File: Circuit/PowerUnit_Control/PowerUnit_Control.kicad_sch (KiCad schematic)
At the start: 25 parts, among them J1 Conn_01x02_Pin, J10 Conn_01x02_Pin, J11 Conn_01x02_Pin, J2 Conn_01x02_Pin, J3 Conn_01x07_Socket, J4 Conn_01x02_Pin, J5 Conn_01x02_Pin, J6 Conn_01x07_Socket, J7 Conn_01x02_Pin, J8 Conn_01x02_Pin, J9 Conn_01x07_Socket, SW1 SW_Toggle_DPDT

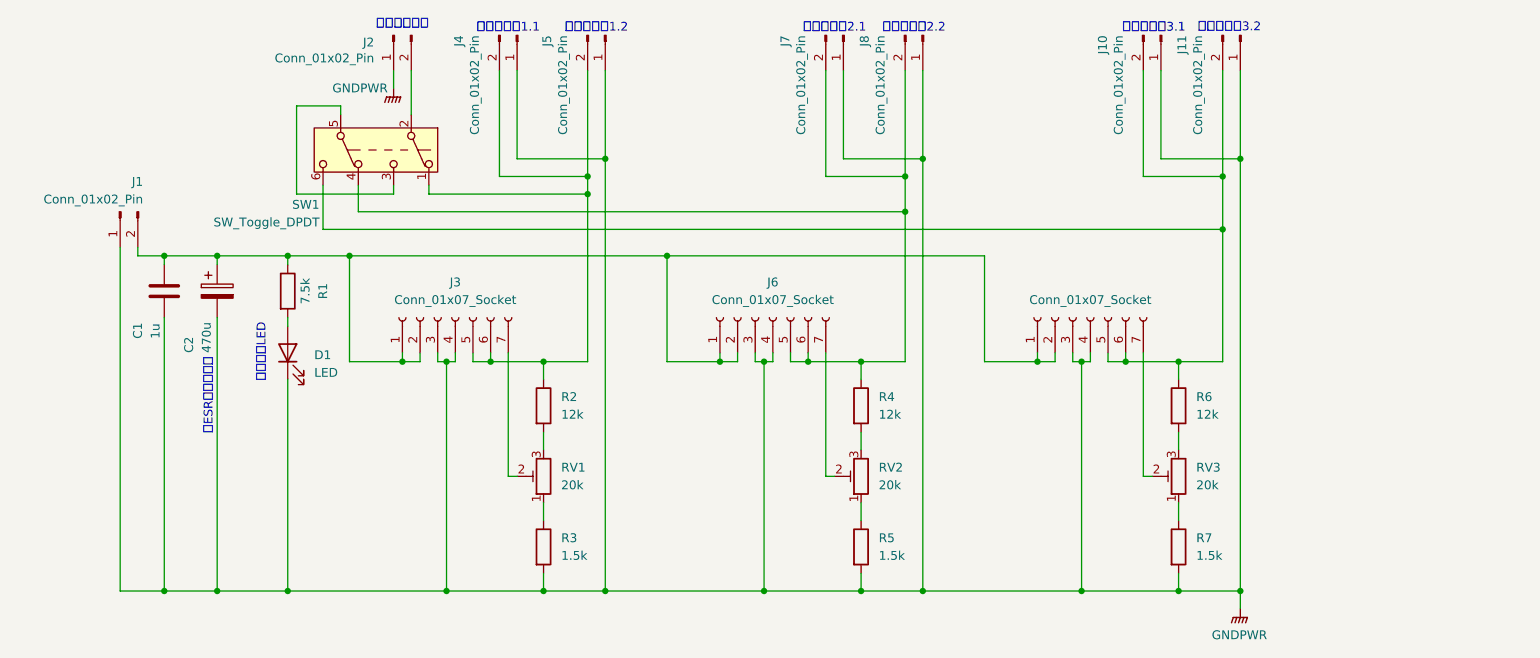
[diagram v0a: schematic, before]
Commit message: 制御電源基板が完成
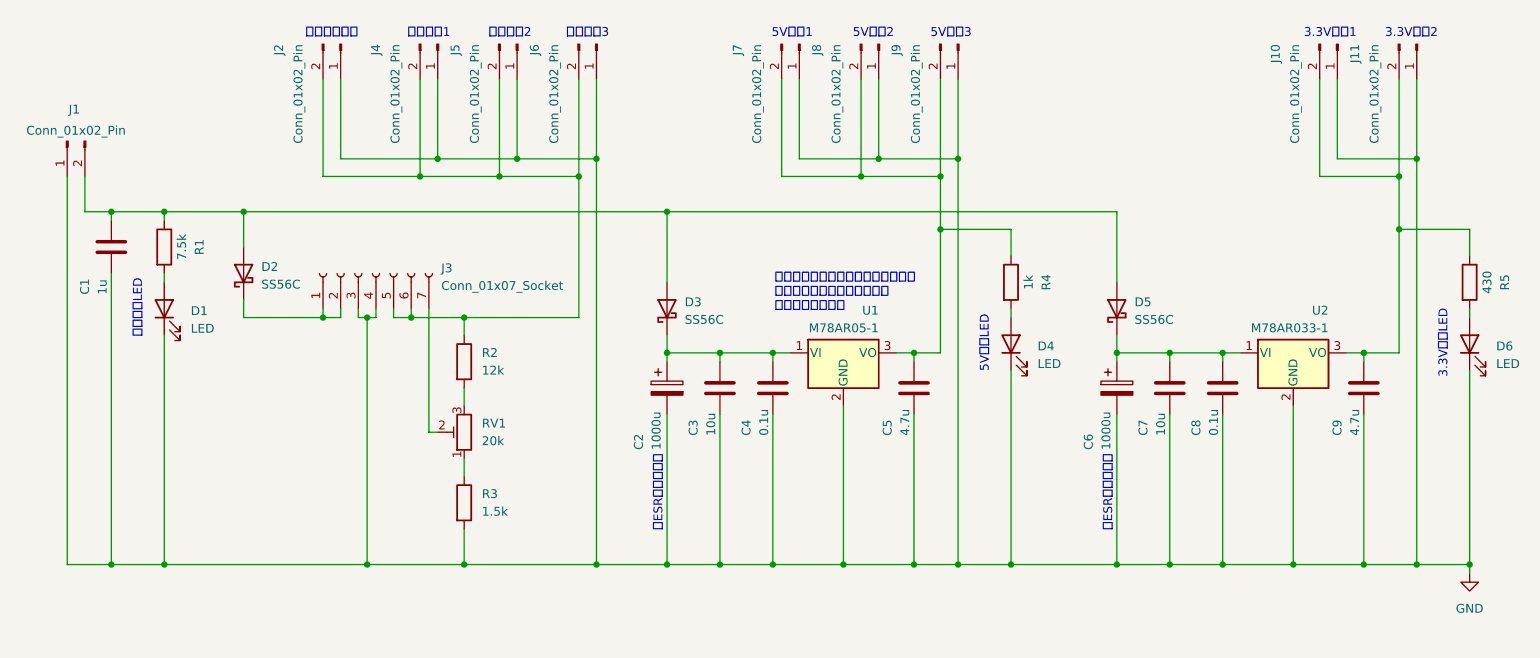
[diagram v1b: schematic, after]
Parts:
- removed J6, J9: Conn_01x07_Socket, OU_Power:YDS512F-Unit, symbol Connector:Conn_01x07_Socket
- removed R6: 12k, Resistor_THT:R_Axial_DIN0207_L6.3mm_D2.5mm_P2.54mm_Vertical, symbol Device:R
- removed R7: 1.5k, Resistor_THT:R_Axial_DIN0207_L6.3mm_D2.5mm_P2.54mm_Vertical, symbol Device:R
- removed RV2, RV3: 20k, OU_Reg:TRIM_3296W-1-250, symbol Device:R_Potentiometer_Trim
- removed SW1: SW_Toggle_DPDT, OU_Switch:1MD6-T1-B1-M1-Q-N-S, symbol Switch:SW_Push_DPDT
- added C3, C7: 10u, Capacitor_SMD:C_1206_3216Metric, symbol Device:C
- added C4, C8: 0.1u, Capacitor_SMD:C_0603_1608Metric, symbol Device:C
- added C5, C9: 4.7u, Capacitor_SMD:C_0805_2012Metric, symbol Device:C
- added C6: 1000u, Capacitor_THT:CP_Radial_D16.0mm_P7.50mm, symbol Device:C_Polarized
- added D2, D3, D5: SS56C, OU_Diode:DIODE_SS56C-HF_CIP, symbol Device:D_Schottky
- added D4, D6: LED, LED_THT:LED_D5.0mm, symbol Device:LED
- added J6: Conn_01x02_Pin, OU_Conn:AMASS_XT30U-F, symbol Connector:Conn_01x02_Pin
- added J9: Conn_01x02_Pin, OU_Conn:Hirose_DF1EC-2P-2.5DSA_1x02_P2.5mm_Vertical, symbol Connector:Conn_01x02_Pin
- added U1: M78AR05-1, OU_Power:M78AR05-1, symbol Regulator_Linear:LM7812_TO220
- added U2: M78AR033-1, OU_Power:M78AR033-1, symbol Regulator_Linear:LM7812_TO220
- C1: footprint Capacitor_THT:C_Disc_D6.0mm_W4.4mm_P5.00mm -> Capacitor_SMD:C_0603_1608Metric; MPN (none) -> C15849; MPN_URL https://akizukidenshi.com/catalog/g/g108150/ -> (none)
- C2: value 470u -> 1000u; footprint Capacitor_THT:CP_Radial_D10.0mm_P5.00mm -> Capacitor_THT:CP_Radial_D16.0mm_P7.50mm; MPN_URL https://akizukidenshi.com/catalog/g/g102719/ -> https://akizukidenshi.com/catalog/g/g108442/
- J1: footprint OU_Conn:AMASS_XT60PW-M -> OU_Conn:AMASS_XT30PW-M; MPN (none) -> XT30PW-M; MPN_URL (none) -> https://akizukidenshi.com/catalog/g/g117949/
- J10, J11, J7, J8: footprint OU_Conn:AMASS_XT30U-F -> OU_Conn:Hirose_DF1EC-2P-2.5DSA_1x02_P2.5mm_Vertical; MPN XT30PW-M -> (none); MPN_URL https://akizukidenshi.com/catalog/g/g117949/ -> (none)
- R2, R3: footprint Resistor_THT:R_Axial_DIN0207_L6.3mm_D2.5mm_P2.54mm_Vertical -> Resistor_SMD:R_0603_1608Metric
- R4: value 12k -> 1k
- R5: value 1.5k -> 430
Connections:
- net at C1.1, J1.2 (Pin_2), R1.1: now also D2.2 (A), D3.2 (A), D5.2 (A); no longer C2.1, J3.1 (Pin_1), J3.2 (Pin_2)
- net at J10.2 (Pin_2), J11.2 (Pin_2): now also R5.1, C9.1, U2.3 (VO)
- net at J7.2 (Pin_2), J8.2 (Pin_2), R4.1: now also C5.1, J9.2 (Pin_2), U1.3 (VO)
- net at J3.5 (Pin_5), J3.6 (Pin_6), J4.2 (Pin_2)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: now also J2.2 (Pin_2), J6.2 (Pin_2)
- net at R4.2: now also D4.2 (A)
- net GNDPWR renamed GND
- net GND: now also C3.2, C4.2, C5.2, C6.2, C7.2, C8.2, C9.2, D4.1 (K), D6.1 (K), J6.1 (Pin_1), J9.1 (Pin_1), U1.2 (GND), U2.2 (GND); no longer R5.2
- new net: C2.1, C3.1, C4.1, D3.1 (K), U1.1 (VI)
- new net: C6.1, C7.1, C8.1, D5.1 (K), U2.1 (VI)
- new net: D2.1 (K), J3.1 (Pin_1), J3.2 (Pin_2)
- new net: D6.2 (A), R5.2
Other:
- note added: "3.3V電源1"
- note added: "3.3V電源2"
- note added: "3.3V電源LED"
- note added: "5V電源1"
- note added: "5V電源2"
- note added: "5V電源3"
- note added: "5V電源LED"
- note added: "リニアレギュレータっぽいですが、 ピン互換があるスイッチング レギュレータです"
- note added: "制御電源LED"
- note added: "汎用電源1"
- note added: "汎用電源2"
- note added: "汎用電源3"
- note removed: "サーボ汎用1.1"
- note removed: "サーボ汎用1.2"
- note removed: "サーボ汎用2.1"
- note removed: "サーボ汎用2.2"
- note removed: "サーボ汎用3.1"
- note removed: "サーボ汎用3.2"
- note removed: "駆動電源LED"
